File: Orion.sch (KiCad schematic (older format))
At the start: 25 parts, among them J1 USB_A, J2 USB_A, J3 USB_A, J4 USB_A, U1 FE1.1s, U2 PRTR5V0U2X, Y1 12MHz

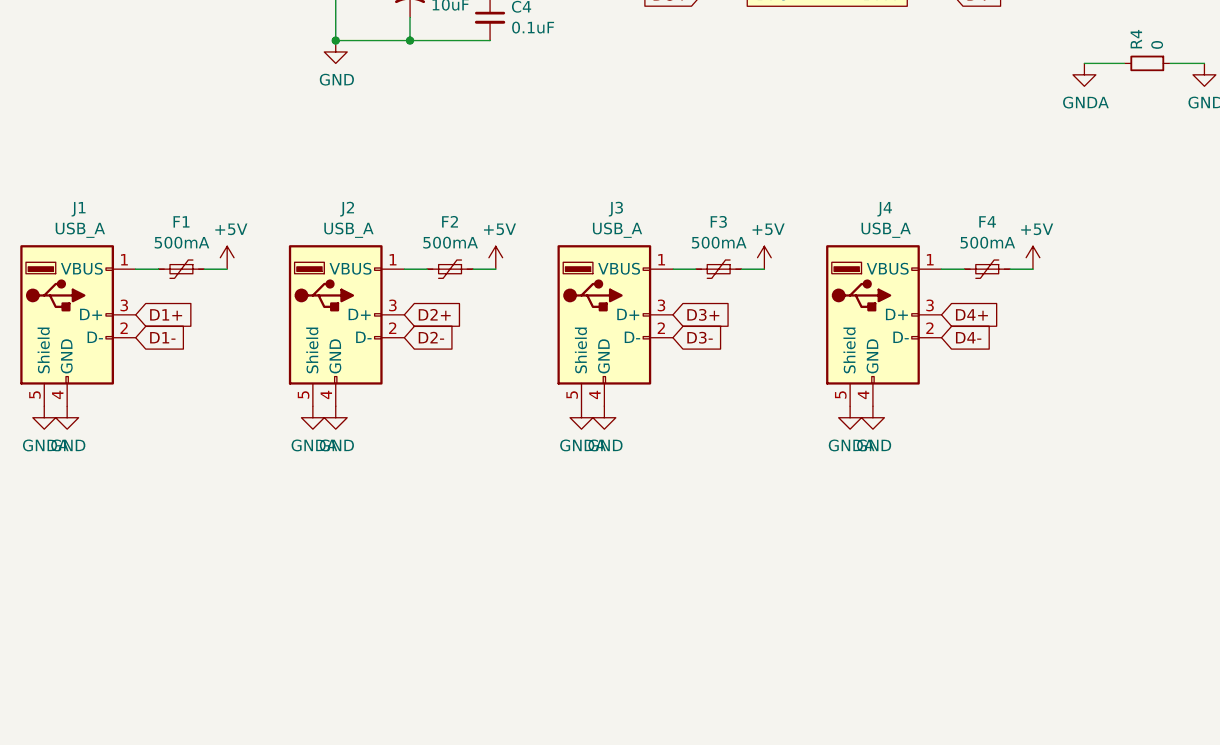
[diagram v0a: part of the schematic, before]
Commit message: Add render
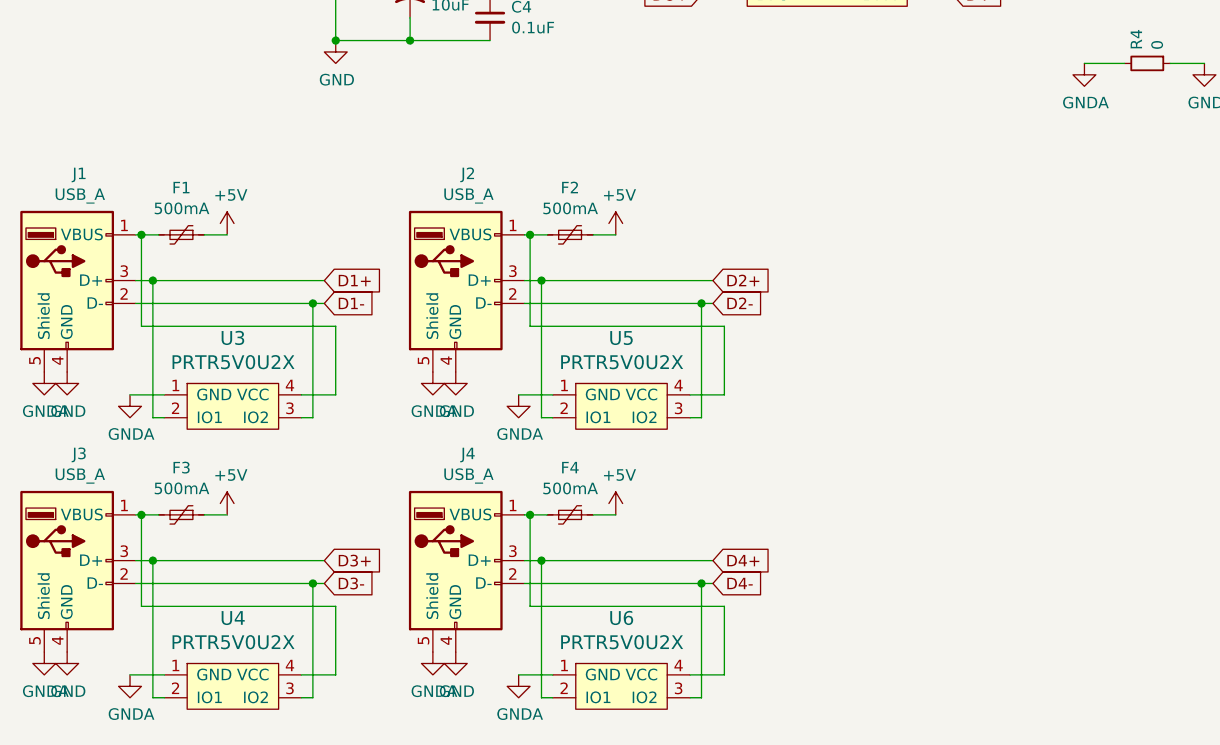
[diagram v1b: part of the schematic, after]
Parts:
- added U3, U4, U5, U6: PRTR5V0U2X, random-keyboard-parts:SOT143B, symbol random-keyboard-parts:PRTR5V0U2X
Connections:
- net D1+: now also U3.2 (IO1)
- net D1-: now also U3.3 (IO2)
- net D2+: now also U5.2 (IO1)
- net D2-: now also U5.3 (IO2)
- net D3+: now also U4.2 (IO1)
- net D3-: now also U4.3 (IO2)
- net D4+: now also U6.2 (IO1)
- net D4-: now also U6.3 (IO2)
- net GNDA: now also U3.1 (GND), U4.1 (GND), U5.1 (GND), U6.1 (GND)
- net at F1.2, J1.1 (VBUS): now also U3.4 (VCC)
- net at F2.2, J2.1 (VBUS): now also U5.4 (VCC)
- net at F3.2, J3.1 (VBUS): now also U4.4 (VCC)
- net at F4.2, J4.1 (VBUS): now also U6.4 (VCC)
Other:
- moved on the sheet: F1, F2, F3, F4, J1, J2, J3, J4
